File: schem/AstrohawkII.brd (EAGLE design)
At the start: 100 x 80 mm, 4 parts, among them J1 RASPBERRYPI-40-PIN-GPIO_PTH_N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

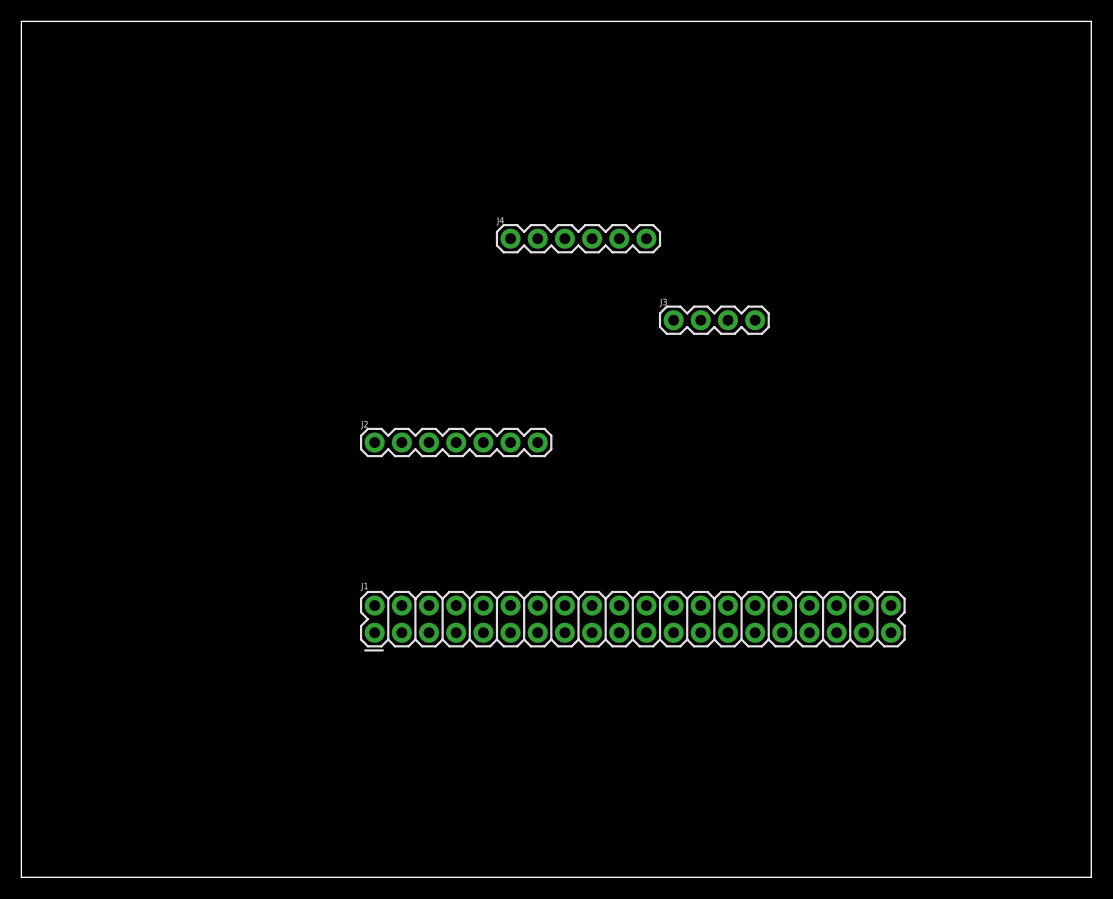
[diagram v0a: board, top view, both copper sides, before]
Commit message: updates eagle schematic and board
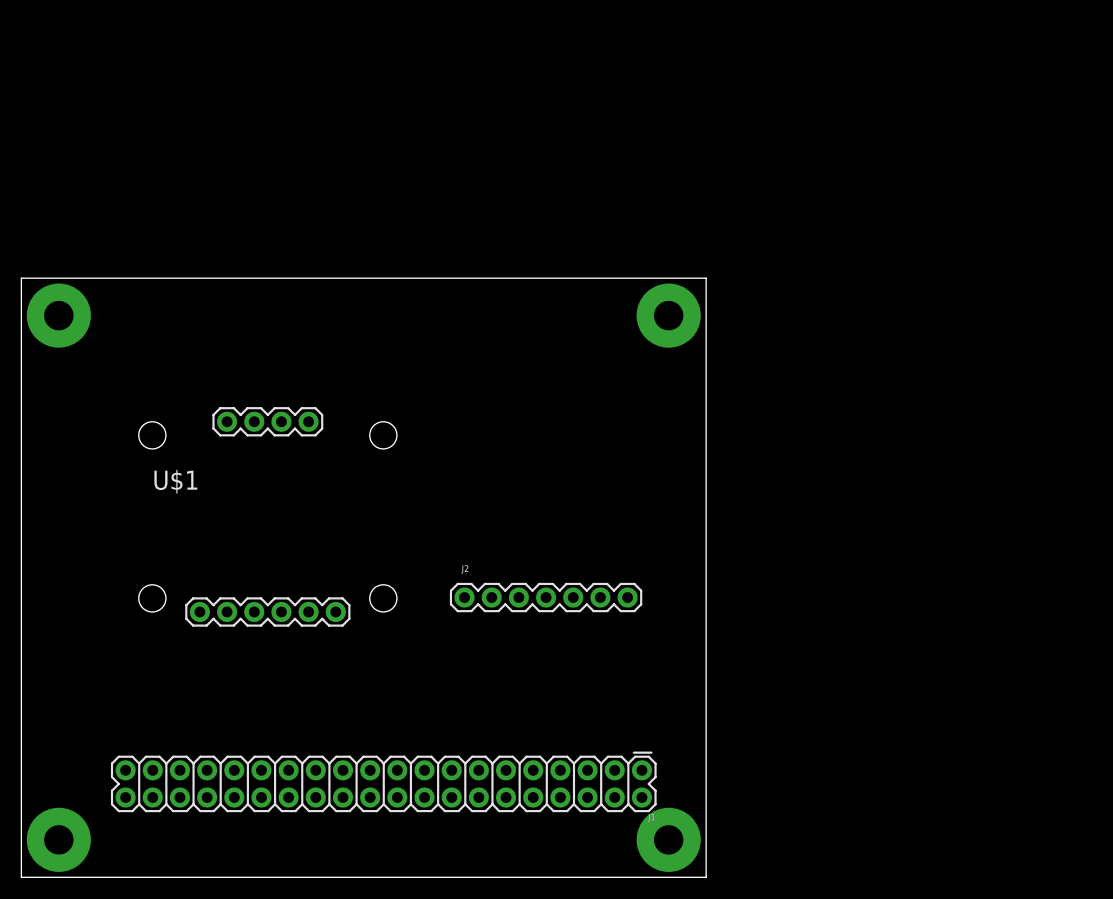
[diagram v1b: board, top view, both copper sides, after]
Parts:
- removed J3: (no value), SparkFun-Connectors:1X04
- removed J4: (no value), SparkFun-Connectors:1X06
- added U$1: BNO055, rocketry:BNO055
- moved J1 28.1 mm to (58.0, 10.0), turned to 180 degrees
- moved J2 16.7 mm to (41.4, 26.1)
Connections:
- removed net 3VO: J2.3, J4.2
- removed net ADR: J3.4
- removed net PS0: J3.1
- removed net PS1: J3.2
- net GND: no longer J4.3
- net INT: now also J1.29; no longer J3.3
- net INT1: now also J1.32
- net INT2: now also J1.33
- net RST: now also J1.31; no longer J4.6
- net SCL: no longer J4.5
- net SDA: no longer J4.4
- net VIN: no longer J4.1
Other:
- board size 100 x 80 mm -> 64 x 56 mm
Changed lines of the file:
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@@
 <setting verticaltext="up"/>
 </settings>
-<grid distance="50" unitdist="mil" unit="mil" style="lines" multiple="1" display="no" altdistance="5" altunitdist="mil" altunit="mil"/>
+<grid distance="1" unitdist="mm" unit="mm" style="lines" multiple="1" display="no" altdistance="0.5" altunitdist="mm" altunit="mm"/>
 <layers>
 <layer number="1" name="Top" color="4" fill="1" visible="yes" active="yes"/>
@@
 <board>
 <plain>
-<wire x1="0" y1="0" x2="100" y2="0" width="0" layer="20"/>
-<wire x1="100" y1="0" x2="100" y2="80" width="0" layer="20"/>
-<wire x1="100" y1="80" x2="0" y2="80" width="0" layer="20"/>
-<wire x1="0" y1="80" x2="0" y2="0" width="0" layer="20"/>
+<wire x1="0" y1="0" x2="64" y2="0" width="0" layer="20"/>
+<wire x1="64" y1="0" x2="64" y2="56" width="0" layer="20"/>
+<wire x1="64" y1="56" x2="0" y2="56" width="0" layer="20"/>
+<wire x1="0" y1="56" x2="0" y2="0" width="0" layer="20"/>
+<dimension x1="3" y1="53" x2="61" y2="53" x3="32" y3="53" textsize="1.778" layer="1"/>
 </plain>
 <attributes>
@@
 </autorouter>
 <elements>
-<element name="J1" library="SparkFun-Connectors" package="2X20" value="RASPBERRYPI-40-PIN-GPIO_PTH_NO_SHROUD" x="33.02" y="22.86" smashed="yes">
-<attribute name="NAME" x="31.75" y="26.924" size="0.6096" layer="25" font="vector" ratio="20"/>
-<attribute name="VALUE" x="31.75" y="20.447" size="0.6096" layer="27" font="vector" ratio="20"/>
+<element name="J1" library="SparkFun-Connectors" package="2X20" value="RASPBERRYPI-40-PIN-GPIO_PTH_NO_SHROUD" x="58" y="10" smashed="yes" rot="R180">
+<attribute name="NAME" x="59.27" y="5.936" size="0.6096" layer="25" font="vector" ratio="20" rot="R180"/>
+<attribute name="VALUE" x="59.27" y="12.413" size="0.6096" layer="27" font="vector" ratio="20" rot="R180"/>
 </element>
-<element name="J2" library="SparkFun-Connectors" package="1X07" value="" x="33.02" y="40.64" smashed="yes">
-<attribute name="MPL3115A2" value="" x="63.5" y="30.48" size="1.778" layer="27" display="off"/>
-<attribute name="NAME" x="31.75" y="42.037" size="0.6096" layer="25" font="vector" ratio="20"/>
-<attribute name="VALUE" x="31.75" y="38.608" size="0.6096" layer="27" font="vector" ratio="20"/>
+<element name="J2" library="SparkFun-Connectors" package="1X07" value="" x="41.42" y="26.15" smashed="yes">
+<attribute name="MPL3115A2" value="" x="71.9" y="15.99" size="1.778" layer="27" display="off"/>
+<attribute name="NAME" x="41.15" y="28.547" size="0.6096" layer="25" font="vector" ratio="20"/>
+<attribute name="VALUE" x="40.15" y="24.118" size="0.6096" layer="27" font="vector" ratio="20"/>
 </element>
-<element name="J3" library="SparkFun-Connectors" package="1X04" value="" x="60.96" y="52.07" smashed="yes">
-<attribute name="BNO055X04" value="" x="83.82" y="34.29" size="1.778" layer="27" display="off"/>
-<attribute name="NAME" x="59.69" y="53.467" size="0.6096" layer="25" font="vector" ratio="20"/>
-<attribute name="PROD_ID" value="CONN-09696" x="83.82" y="34.29" size="1.778" layer="27" display="off"/>
-<attribute name="VALUE" x="59.69" y="50.038" size="0.6096" layer="27" font="vector" ratio="20"/>
-</element>
-<element name="J4" library="SparkFun-Connectors" package="1X06" value="" x="45.72" y="59.69" smashed="yes">
-<attribute name="BNO055X06" value="" x="73.66" y="45.72" size="1.778" layer="27" display="off"/>
-<attribute name="NAME" x="44.45" y="61.087" size="0.6096" layer="25" font="vector" ratio="20"/>
-<attribute name="PROD_ID" value="CONN-08437" x="73.66" y="45.72" size="1.778" layer="27" display="off"/>
-<attribute name="VALUE" x="44.45" y="57.658" size="0.6096" layer="27" font="vector" ratio="20"/>
+<element name="U$1" library="rocketry" package="BNO055" value="BNO055" x="9.7" y="23.53" smashed="yes">
+<attribute name="NAME" x="12.24" y="36.23" size="1.778" layer="25"/>
+<attribute name="VALUE" x="12.24" y="29.88" size="1.778" layer="27"/>
 </element>
 </elements>
@@
 <contactref element="J1" pad="1"/>
 <contactref element="J1" pad="17"/>
-<wire x1="53.34" y1="22.86" x2="33.02" y2="22.86" width="0" layer="19" extent="1-1"/>
-</signal>
-<signal name="PS0">
-<contactref element="J3" pad="1"/>
-</signal>
-<signal name="PS1">
-<contactref element="J3" pad="2"/>
-</signal>
-<signal name="INT">
-<contactref element="J3" pad="3"/>
-</signal>
-<signal name="ADR">
-<contactref element="J3" pad="4"/>
+<wire x1="37.68" y1="10" x2="58" y2="10" width="0" layer="19" extent="1-1"/>
 </signal>
 <signal name="VIN">
 <contactref element="J2" pad="1"/>
-<contactref element="J4" pad="1"/>
 <contactref element="J1" pad="2"/>
 <contactref element="J1" pad="4"/>
-<wire x1="35.56" y1="25.4" x2="33.02" y2="25.4" width="0" layer="19" extent="1-1"/>
-<wire x1="33.02" y1="40.64" x2="35.56" y2="25.4" width="0" layer="19" extent="1-1"/>
-<wire x1="45.72" y1="59.69" x2="33.02" y2="40.64" width="0" layer="19" extent="1-1"/>
+<wire x1="58" y1="7.46" x2="41.42" y2="26.15" width="0" layer="19" extent="1-1"/>
+<wire x1="55.46" y1="7.46" x2="58" y2="7.46" width="0" layer="19" extent="1-1"/>
 </signal>
 <signal name="GND">
 <contactref element="J2" pad="2"/>
-<contactref element="J4" pad="3"/>
 <contactref element="J1" pad="6"/>
 <contactref element="J1" pad="9"/>
@@
 <contactref element="J1" pad="34"/>
 <contactref element="J1" pad="39"/>
-<wire x1="43.18" y1="22.86" x2="38.1" y2="25.4" width="0" layer="19" extent="1-1"/>
-<wire x1="48.26" y1="25.4" x2="43.18" y2="22.86" width="0" layer="19" extent="1-1"/>
-<wire x1="55.88" y1="25.4" x2="48.26" y2="25.4" width="0" layer="19" extent="1-1"/>
-<wire x1="63.5" y1="22.86" x2="55.88" y2="25.4" width="0" layer="19" extent="1-1"/>
-<wire x1="68.58" y1="25.4" x2="63.5" y2="22.86" width="0" layer="19" extent="1-1"/>
-<wire x1="35.56" y1="40.64" x2="68.58" y2="25.4" width="0" layer="19" extent="1-1"/>
-<wire x1="73.66" y1="25.4" x2="68.58" y2="25.4" width="0" layer="19" extent="1-1"/>
-<wire x1="50.8" y1="59.69" x2="35.56" y2="40.64" width="0" layer="19" extent="1-1"/>
-<wire x1="81.28" y1="22.86" x2="73.66" y2="25.4" width="0" layer="19" extent="1-1"/>
-</signal>
-<signal name="3VO">
-<contactref element="J2" pad="3"/>
-<contactref element="J4" pad="2"/>
-<wire x1="48.26" y1="59.69" x2="38.1" y2="40.64" width="0" layer="19" extent="1-1"/>
+<wire x1="17.36" y1="7.46" x2="9.74" y2="10" width="0" layer="19" extent="1-1"/>
+<wire x1="22.44" y1="7.46" x2="17.36" y2="7.46" width="0" layer="19" extent="1-1"/>
+<wire x1="27.52" y1="10" x2="22.44" y2="7.46" width="0" layer="19" extent="1-1"/>
+<wire x1="35.14" y1="7.46" x2="27.52" y2="10" width="0" layer="19" extent="1-1"/>
+<wire x1="42.76" y1="7.46" x2="35.14" y2="7.46" width="0" layer="19" extent="1-1"/>
+<wire x1="47.84" y1="10" x2="42.76" y2="7.46" width="0" layer="19" extent="1-1"/>
+<wire x1="52.92" y1="7.46" x2="47.84" y2="10" width="0" layer="19" extent="1-1"/>
+<wire x1="43.96" y1="26.15" x2="52.92" y2="7.46" width="0" layer="19" extent="1-1"/>
 </signal>
 <signal name="INT2">
 <contactref element="J2" pad="4"/>
+<contactref element="J1" pad="33"/>
+<wire x1="49.04" y1="26.15" x2="17.36" y2="10" width="0" layer="19" extent="1-1"/>
 </signal>
 <signal name="INT1">
 <contactref element="J2" pad="5"/>
+<contactref element="J1" pad="32"/>
+<wire x1="51.58" y1="26.15" x2="19.9" y2="7.46" width="0" layer="19" extent="1-1"/>
 </signal>
 <signal name="SCL">
 <contactref element="J2" pad="6"/>
-<contactref element="J4" pad="5"/>
 <contactref element="J1" pad="5"/>
-<wire x1="45.72" y1="40.64" x2="38.1" y2="22.86" width="0" layer="19" extent="1-1"/>
-<wire x1="55.88" y1="59.69" x2="45.72" y2="40.64" width="0" layer="19" extent="1-1"/>
+<wire x1="52.92" y1="10" x2="54.12" y2="26.15" width="0" layer="19" extent="1-1"/>
 </signal>
 <signal name="SDA">
 <contactref element="J2" pad="7"/>
-<contactref element="J4" pad="4"/>
 <contactref element="J1" pad="3"/>
-<wire x1="53.34" y1="59.69" x2="35.56" y2="22.86" width="0" layer="19" extent="1-1"/>
-<wire x1="48.26" y1="40.64" x2="53.34" y2="59.69" width="0" layer="19" extent="1-1"/>
+<wire x1="55.46" y1="10" x2="56.66" y2="26.15" width="0" layer="19" extent="1-1"/>
+</signal>
+<signal name="INT">
+<contactref element="J1" pad="29"/>
 </signal>
 <signal name="RST">
-<contactref element="J4" pad="6"/>
+<contactref element="J1" pad="31"/>
+</signal>
+<signal name="N$1">
+<via x="3.5" y="52.5" extent="1-16" drill="2.75" diameter="6"/>
+</signal>
+<signal name="N$2">
+<via x="3.5" y="3.5" extent="1-16" drill="2.75" diameter="6"/>
+</signal>
+<signal name="N$3">
+<via x="60.5" y="3.5" extent="1-16" drill="2.75" diameter="6"/>
+</signal>
+<signal name="N$4">
+<via x="60.5" y="52.5" extent="1-16" drill="2.75" diameter="6"/>
 </signal>
 </signals>
